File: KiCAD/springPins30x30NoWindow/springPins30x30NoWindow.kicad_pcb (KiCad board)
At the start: 2 copper layers, 30 x 30 mm, 24 parts, among them J1 CONN_01X03, J2 CONN_01X03, J3 CONN_01X03, J4 CONN_01X03, J5 CONN_01X03, J6 CONN_01X03, J7 CONN_01X03, J8 CONN_01X03

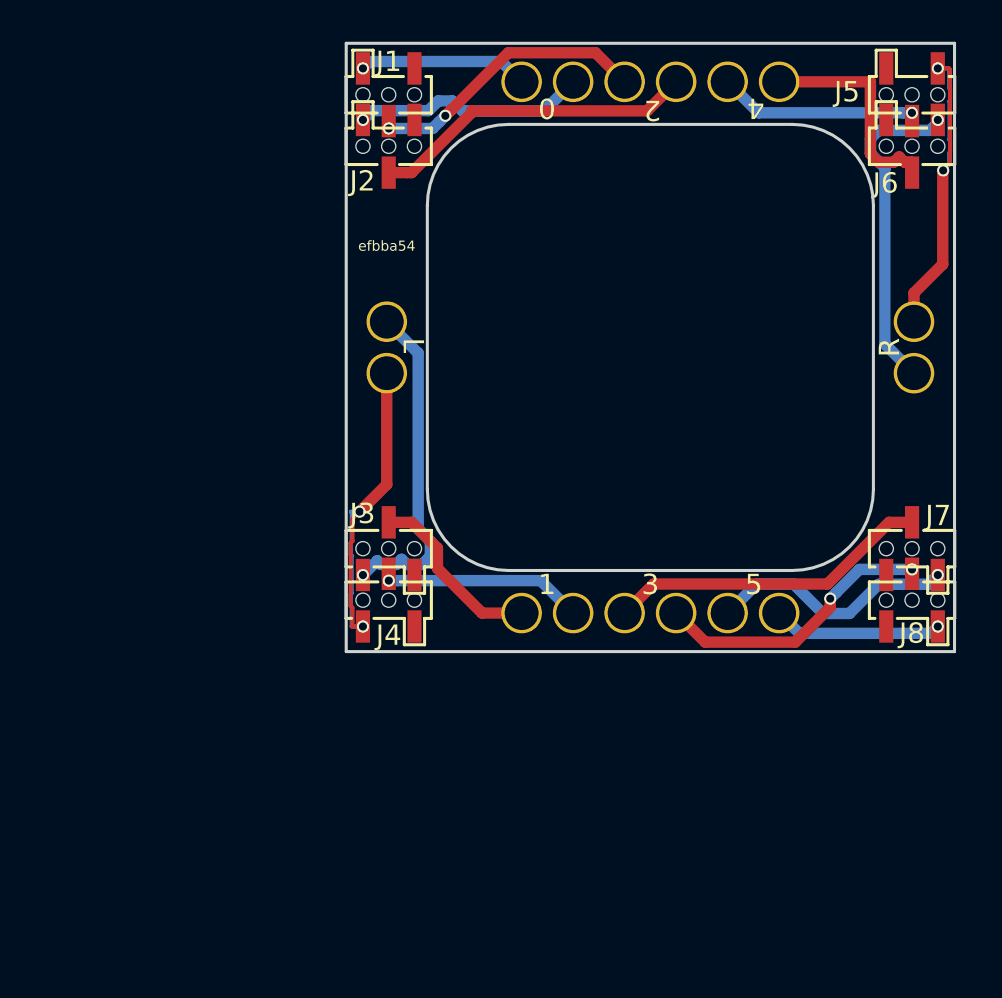
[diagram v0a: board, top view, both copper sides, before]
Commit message: nowindow pin boards done
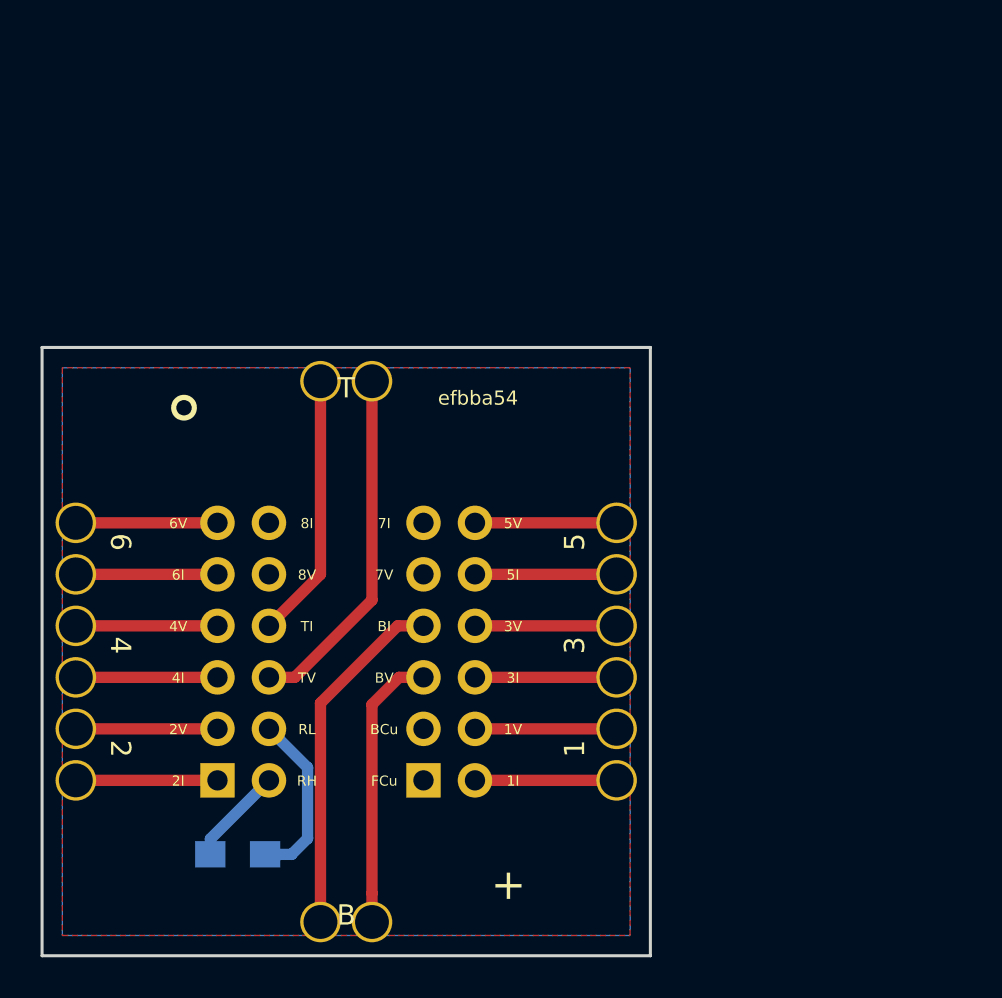
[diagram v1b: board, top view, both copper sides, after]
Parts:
- removed J3, J4, J5, J6, J7, J8: CONN_01X03, myParts:M50-3130342
- removed TP1, TP13, TP14, TP2: TEST, myParts:S25-022+P25-4023
- added R1: 200k, Resistors_SMD:R_0805_HandSoldering, B.Cu at (-5.35, 10.0)
- added TP17: TEST, myParts:S25-022+P25-4023, F.Cu at (13.3, -1.27)
- added TP18: TEST, myParts:S25-022+P25-4023, F.Cu at (13.3, 1.27)
- added TP19: TEST, myParts:S25-022+P25-4023, F.Cu at (13.3, 3.81)
- added TP20: TEST, myParts:S25-022+P25-4023, F.Cu at (13.3, 6.35)
- J1, J2: value CONN_01X03 -> CONN_02X06; footprint myParts:M50-3130342 -> Pin_Headers:Pin_Header_Straight_2x06_Pitch2.54mm; moved to B.Cu
- moved TP7 41.8 mm to (-13.3, 3.81)
- moved TP5 36.4 mm to (-13.3, -1.27)
- moved J1 34.6 mm to (-6.35, 6.35)
- moved J2 31.4 mm to (3.81, 6.35)
- moved TP3 30.9 mm to (-13.3, -6.35)
- moved TP8 28.3 mm to (-13.3, 6.35)
- moved TP6 24.7 mm to (-13.3, 1.27)
- moved TP10 23.2 mm to (-1.27, 13.3)
- moved TP12 23.2 mm to (1.27, 13.3)
- moved TP11 22.9 mm to (1.27, -13.3)
- moved TP9 22.9 mm to (-1.27, -13.3)
- moved TP4 22.1 mm to (-13.3, -3.81)
- moved TP15 17.7 mm to (13.3, -6.35)
- moved TP16 17.7 mm to (13.3, -3.81)
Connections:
- net /MOSI renamed BCu
- J1 pad 1: 0_V -> /I2
- J1 pad 2: 2_V -> /RH
- J1 pad 3: /MISO -> /V2
- J2 pad 1: 0_I -> FCu
- J2 pad 2: 2_I -> /I1
- TP10 pad 1: 3_V -> /IB
- TP11 pad 1: 4_V -> /VT
- TP12 pad 1: 5_I -> /VB
- TP15 pad 1: R_V -> /V5
- TP16 pad 1: R_I -> /I5
- TP3 pad 1: 0_V -> /V6
- TP4 pad 1: 1_I -> /I6
- TP5 pad 1: 0_I -> /V4
- TP6 pad 1: 1_V -> /I4
- TP7 pad 1: 2_V -> /V2
- TP8 pad 1: 3_I -> /I2
- TP9 pad 1: 2_I -> /IT
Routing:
- net L_V: track 20.6 -> 0.00 mm, vias 2 -> 0
- net R_V: track 19.6 -> 0.00 mm, vias 2 -> 0
- net /VT: track 0.00 -> 17.5 mm
- net /IB: track 0.00 -> 17.5 mm
- net L_I: track 16.5 -> 0.00 mm, vias 1 -> 0
- net R_I: track 16.2 -> 0.00 mm, vias 1 -> 0
- net 2_I: track 16.1 -> 0.00 mm
- net 3_I: track 16.0 -> 0.00 mm
- net 3_V: track 14.0 -> 0.00 mm, vias 2 -> 0
- net /VB: track 0.00 -> 13.8 mm
- net 2_V: track 13.8 -> 0.00 mm, vias 2 -> 0
- net /IT: track 0.00 -> 13.1 mm
- net 5_I: track 12.3 -> 0.00 mm, vias 1 -> 0
- net 0_I: track 11.5 -> 0.00 mm, vias 1 -> 0
- net 4_I: track 11.0 -> 0.00 mm
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- added copper zone on B.Cu, net BCu
- added copper zone on F.Cu, net FCu
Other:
- outline, holes or cut-outs redrawn
- board text added: "+"
- board text added: "1I"
- board text added: "1V"
- board text added: "2I"
- board text added: "2V"
- board text added: "3I"
- board text added: "3V"
- board text added: "4I"
- board text added: "4V"
- board text added: "5I"
- board text added: "5V"
- board text added: "6"
- board text added: "6I"
- board text added: "6V"
- board text added: "7I"
- board text added: "7V"
- board text added: "8I"
- board text added: "8V"
- board text added: "B"
- board text added: "BCu"
- board text added: "BI"
- board text added: "BV"
- board text added: "FCu"
- board text added: "RH"
- board text added: "RL"
- board text added: "T"
- board text added: "TI"
- board text added: "TV"
- board text added: "°"
- board text removed: "0"
- board text removed: "L"
- board text removed: "R"
